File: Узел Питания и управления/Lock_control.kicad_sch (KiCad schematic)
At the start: 0 parts

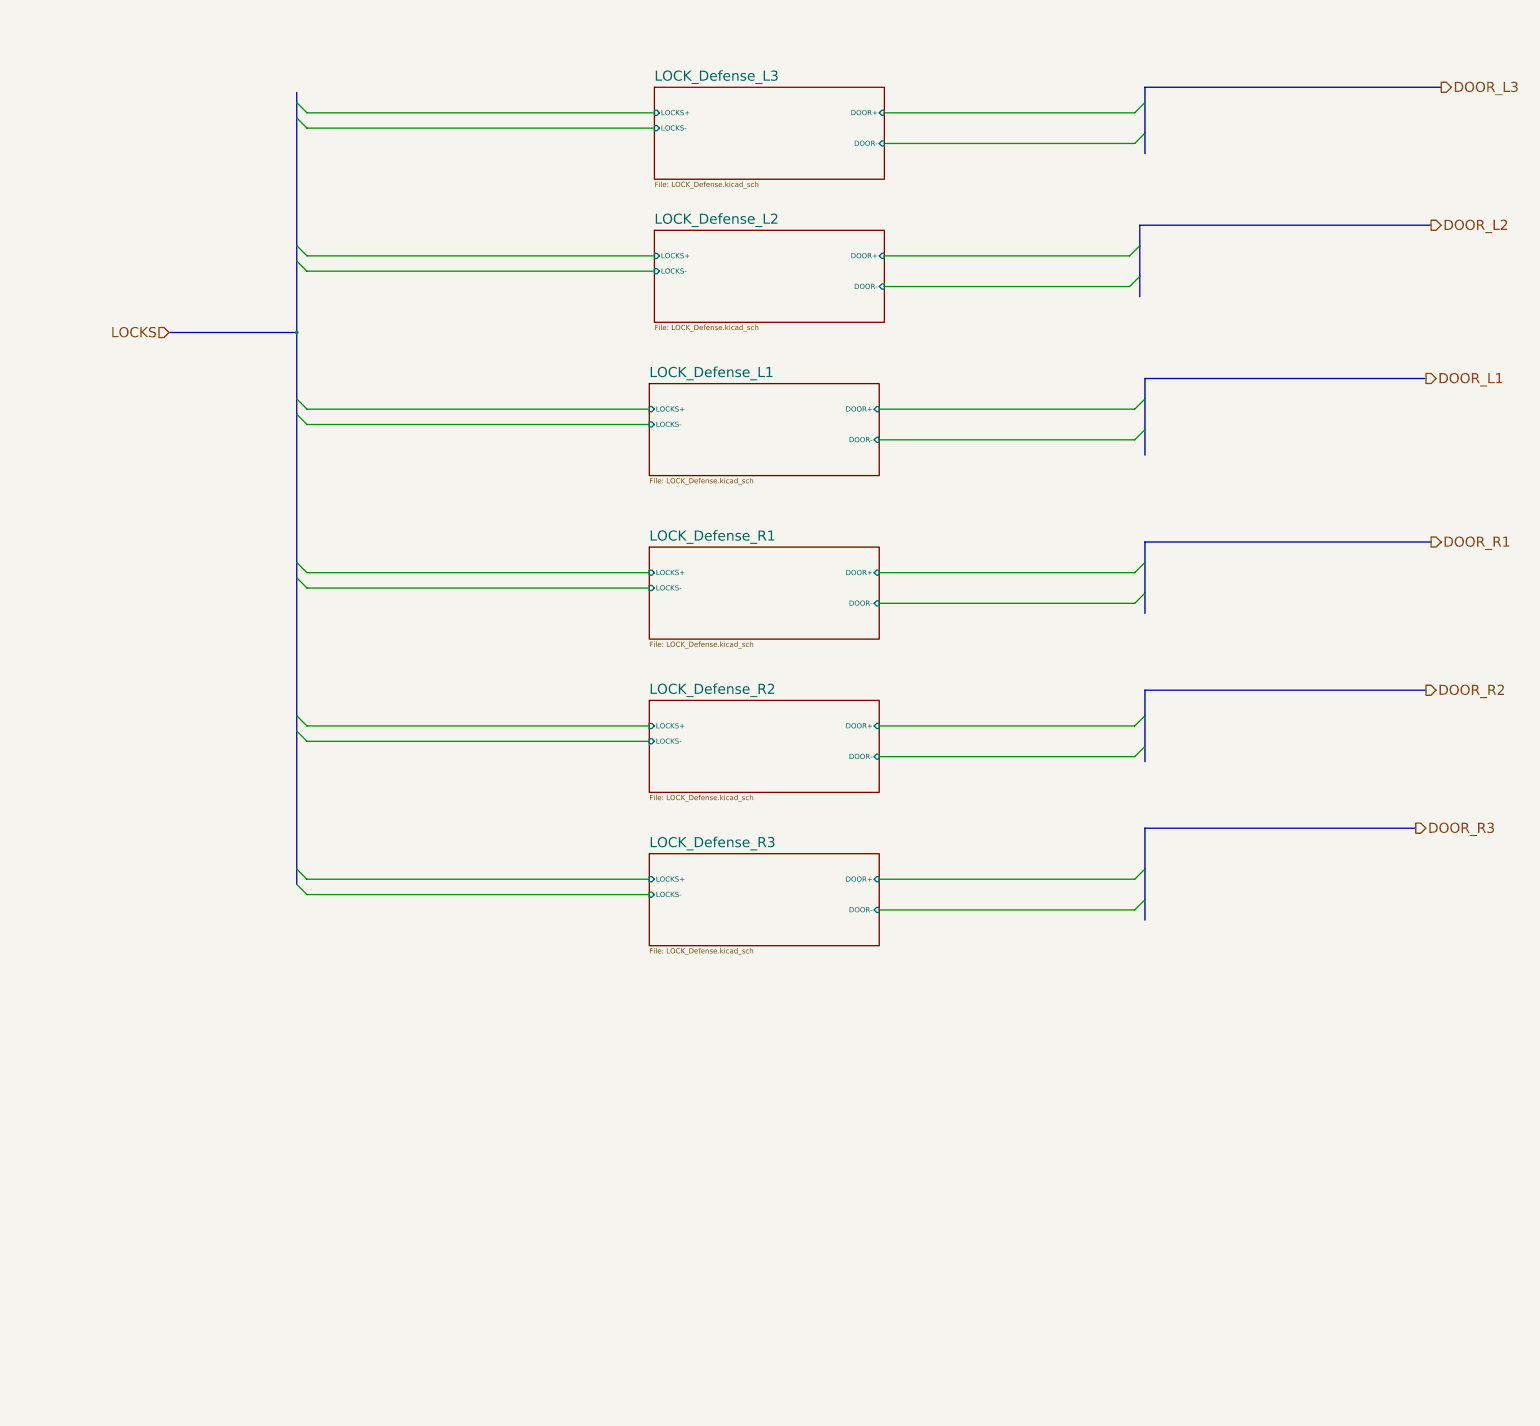
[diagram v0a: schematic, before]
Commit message: update schemas
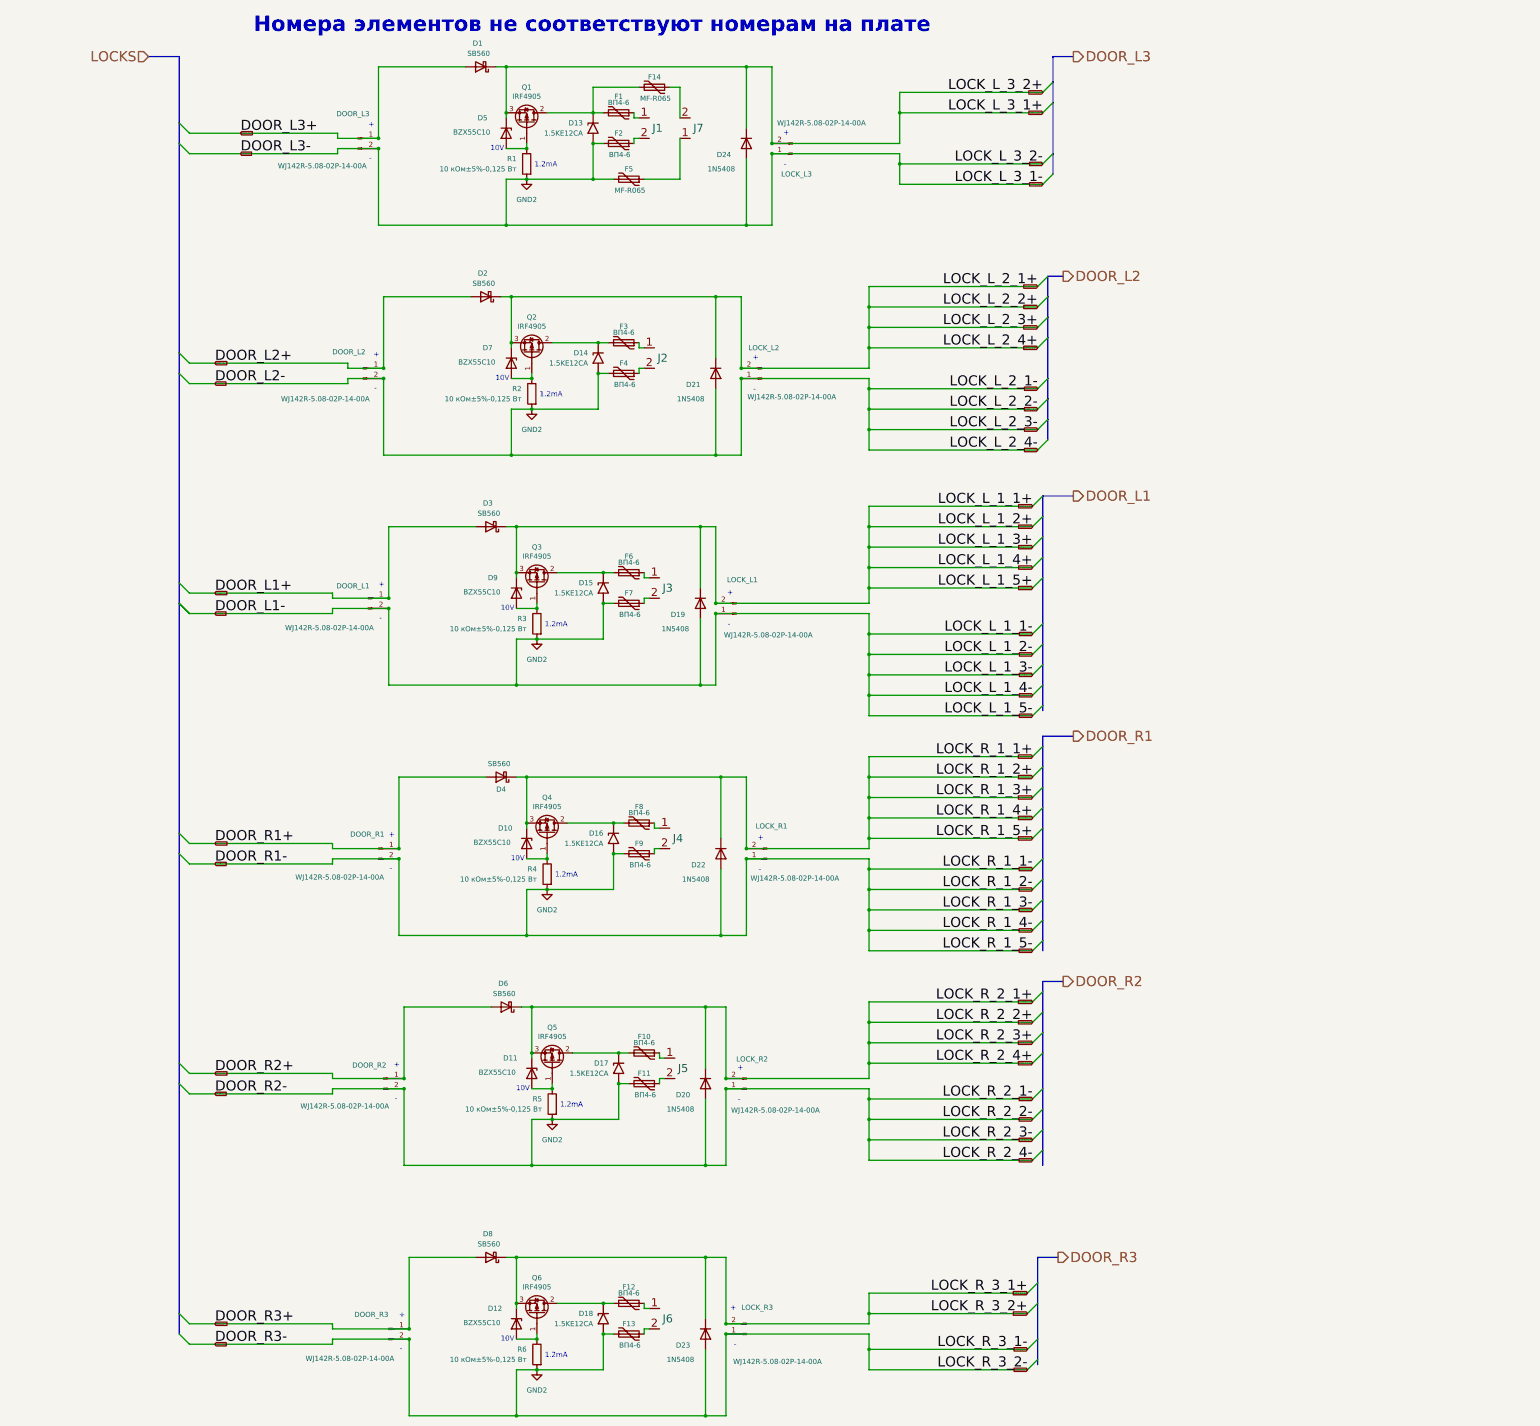
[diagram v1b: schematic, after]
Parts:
- added D1, D2, D3, D4, D6, D8: SB560, Diode_THT:D_DO-201AD_P10.16mm_Horizontal, symbol Diode:1N5822
- added D10, D11, D12, D5, D7, D9: BZX55C10, Diode_THT:D_DO-35_SOD27_P5.08mm_Vertical_AnodeUp, symbol Diode:BZX384xxxx
- added D13, D14, D15, D16, D17, D18: 1.5KE12CA, Diode_THT:D_DO-201AD_P10.16mm_Horizontal, symbol Diode:SM6T12A
- added D19, D20, D21, D22, D23, D24: 1N5408, Diode_THT:D_DO-201AD_P15.24mm_Horizontal, symbol Diode:1N5408
- added DOOR_L1, DOOR_L2, DOOR_L3, DOOR_R1, DOOR_R2, DOOR_R3, LOCK_L1, LOCK_L2, LOCK_L3, LOCK_R1, LOCK_R2, LOCK_R3: WJ142R-5.08-02P-14-00A, Connector:DG141R-02, symbol Connector:Conn_01x02_Pin
- added F1, F10, F11, F12, F13, F2, F3, F4, F6, F7, F8, F9: ВП4-6, Diode_THT:D_DO-201AD_P12.70mm_Horizontal, symbol Device:Polyfuse
- added F14, F5: MF-R065, Fuse:Fuse_Bourns_MF-RG300, symbol Device:Polyfuse
- added J1, J2, J3, J4, J5, J6, J7: ~, Connector_Phoenix_MSTB:PhoenixContact_MSTBVA_2,5_2-G-5,08_1x02_P5.08mm_Vertical, symbol Connector:Conn_01x02_(wide)
- added Q1, Q2, Q3, Q4, Q5, Q6: IRF4905, Package_TO_SOT_THT:TO-220-3_Horizontal_TabDown, symbol Transistor_FET:IRF4905
- added R1, R2, R3, R4, R5, R6: 10 кОм±5%-0,125 Вт, Resistor_THT:R_Axial_DIN0414_L11.9mm_D4.5mm_P15.24mm_Horizontal, symbol Device:R
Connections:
- new net: F5.1, J7.1
- new net: F1.1, J1.1
- new net: F2.1, J1.2
- new net: D12.2 (A), Q6.1 (G), R6.1
- new net: D18.1 (A1), F12.2, Q6.2 (D)
- new net: F7.1, J3.2
- new net: F3.1, J2.1
- new net: F4.1, J2.2
- new net: F14.1, J7.2
- new net: F9.1, J4.2
- new net: F6.1, J3.1
- new net: D15.1 (A1), F6.2, Q3.2 (D)
- new net: D5.2 (A), Q1.1 (G), R1.1
- new net: D7.2 (A), Q2.1 (G), R2.1
- new net: D11.2 (A), Q5.1 (G), R5.1
- new net: D10.2 (A), Q4.1 (G), R4.1
- new net: D16.1 (A1), F8.2, Q4.2 (D)
- new net: D13.1 (A1), F1.2, F14.2, Q1.2 (D)
- new net: F12.1, J6.1
- new net: F13.1, J6.2
- new net: F10.1, J5.1
- new net: D17.1 (A1), F10.2, Q5.2 (D)
- new net: D9.2 (A), Q3.1 (G), R3.1
- new net: F8.1, J4.1
- new net: D14.1 (A1), F3.2, Q2.2 (D)
- new net: F11.1, J5.2
- new net DOOR_L2+: D2.2 (A), DOOR_L2.1 (Pin_1)
- new net DOOR_L3+: D1.2 (A), D3.2 (A), DOOR_L1.1 (Pin_1), DOOR_L3.1 (Pin_1)
- new net DOOR_R1+: D4.2 (A), DOOR_R1.1 (Pin_1)
- new net DOOR_R2+: D6.2 (A), DOOR_R2.1 (Pin_1)
- new net DOOR_R3+: D8.2 (A), DOOR_R3.1 (Pin_1)
- new net GND2: D13.2 (A2), D14.2 (A2), D15.2 (A2), D16.2 (A2), D17.2 (A2), D18.2 (A2), D19.2 (A), D20.2 (A), D21.2 (A), D22.2 (A), D23.2 (A), D24.2 (A), DOOR_L1.2 (Pin_2), DOOR_L2.2 (Pin_2), DOOR_L3.2 (Pin_2), DOOR_R1.2 (Pin_2), DOOR_R2.2 (Pin_2), DOOR_R3.2 (Pin_2), F11.2, F13.2, F2.2, F4.2, F5.2, F7.2, F9.2, LOCK_L1.1 (Pin_1), LOCK_L2.1 (Pin_1), LOCK_L3.1 (Pin_1), LOCK_R1.1 (Pin_1), LOCK_R2.1 (Pin_1), LOCK_R3.1 (Pin_1), R1.2, R2.2, R3.2, R4.2, R5.2, R6.2
- new net LOCK_L_1_1+: D19.1 (K), D3.1 (K), D9.1 (K), LOCK_L1.2 (Pin_2), Q3.3 (S)
- new net LOCK_L_2_1+: D2.1 (K), D21.1 (K), D7.1 (K), LOCK_L2.2 (Pin_2), Q2.3 (S)
- new net LOCK_L_3_1+: D1.1 (K), D24.1 (K), D5.1 (K), LOCK_L3.2 (Pin_2), Q1.3 (S)
- new net LOCK_R_1_1+: D10.1 (K), D22.1 (K), D4.1 (K), LOCK_R1.2 (Pin_2), Q4.3 (S)
- new net LOCK_R_2_1+: D11.1 (K), D20.1 (K), D6.1 (K), LOCK_R2.2 (Pin_2), Q5.3 (S)
- new net LOCK_R_3_1+: D12.1 (K), D23.1 (K), D8.1 (K), LOCK_R3.2 (Pin_2), Q6.3 (S)
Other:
- removed sheet LOCK_Defense_L1
- removed sheet LOCK_Defense_L2
- removed sheet LOCK_Defense_L3
- removed sheet LOCK_Defense_R1
- removed sheet LOCK_Defense_R2
- removed sheet LOCK_Defense_R3
- note added: "+"
- note added: "-"
- note added: "1.2mA"
- note added: "10V"
- note added: "Номера элементов не соответствуют номерам на плате"
